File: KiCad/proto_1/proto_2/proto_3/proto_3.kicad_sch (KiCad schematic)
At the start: 10 parts

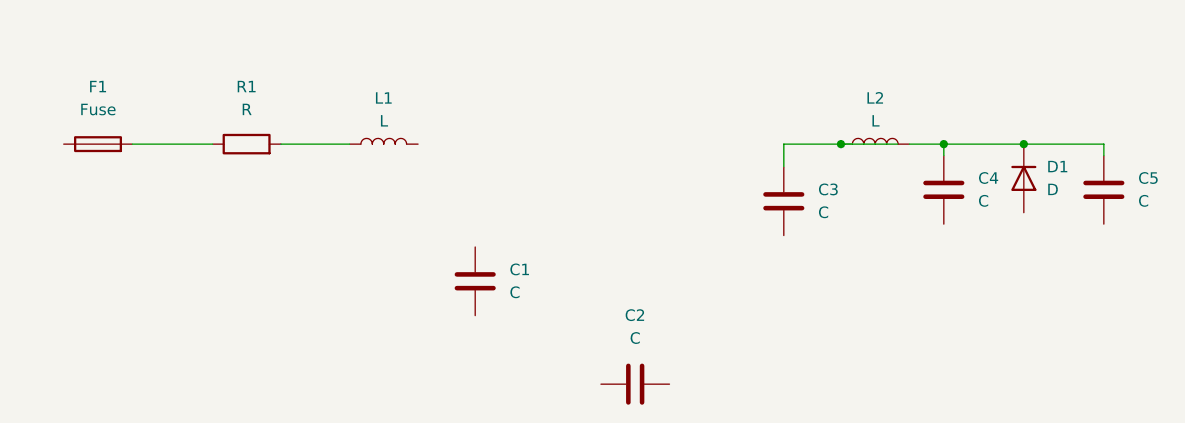
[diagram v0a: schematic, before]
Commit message: more work on proto3
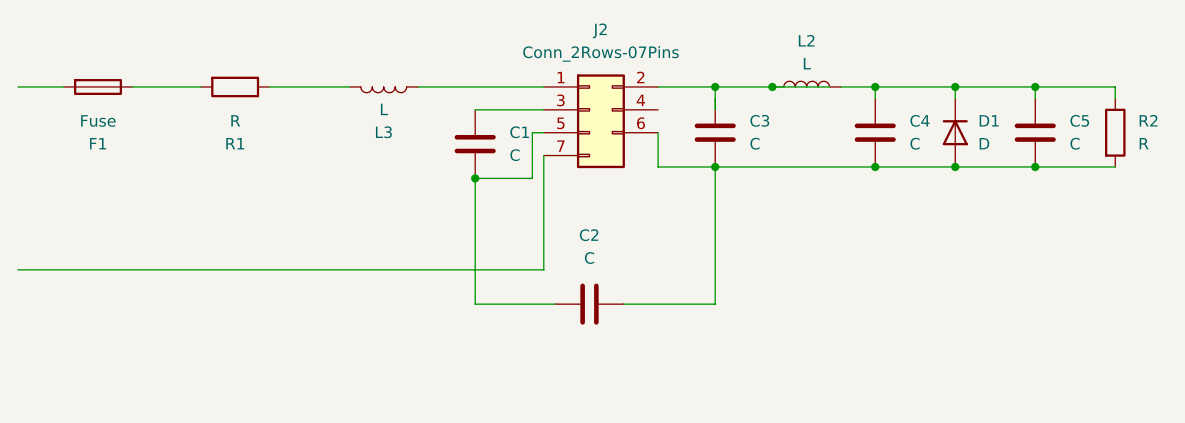
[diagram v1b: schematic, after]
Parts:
- removed L1: L, symbol Device:L
- added J2: Conn_2Rows-07Pins, symbol Connector_Generic:Conn_2Rows-07Pins
- added L3: L, symbol Device:L
- added R2: R, symbol Device:R
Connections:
- net at C4.1, C5.1, D1.1 (K)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: now also R2.1
- net at C4.2: now also C2.2, C3.2, C5.2, D1.2 (A), J2.6 (Pin_6), R2.2
- net at C2.1: now also C1.2, J2.5 (Pin_5)
- net at L2.1: now also J2.2 (Pin_2); no longer C3.1
- net at R1.1: now also L3.2; no longer F1.2
- net at R1.2: now also F1.1
- net at C1.1: now also J2.3 (Pin_3)
- new net: J2.1 (Pin_1), L3.1
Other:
- moved on the sheet: C1, C2, C3, C4, C5, D1, F1, L2, R1
